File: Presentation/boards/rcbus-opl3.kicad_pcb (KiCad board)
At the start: 2 copper layers, 100 x 50 mm, 34 parts, among them CON1 SJ1-3523N, P1 RC2014 BUS, U1 74HCT688, U2 YMF262, U3 YAC512, U4 TL074, Y1 SG-8002CA

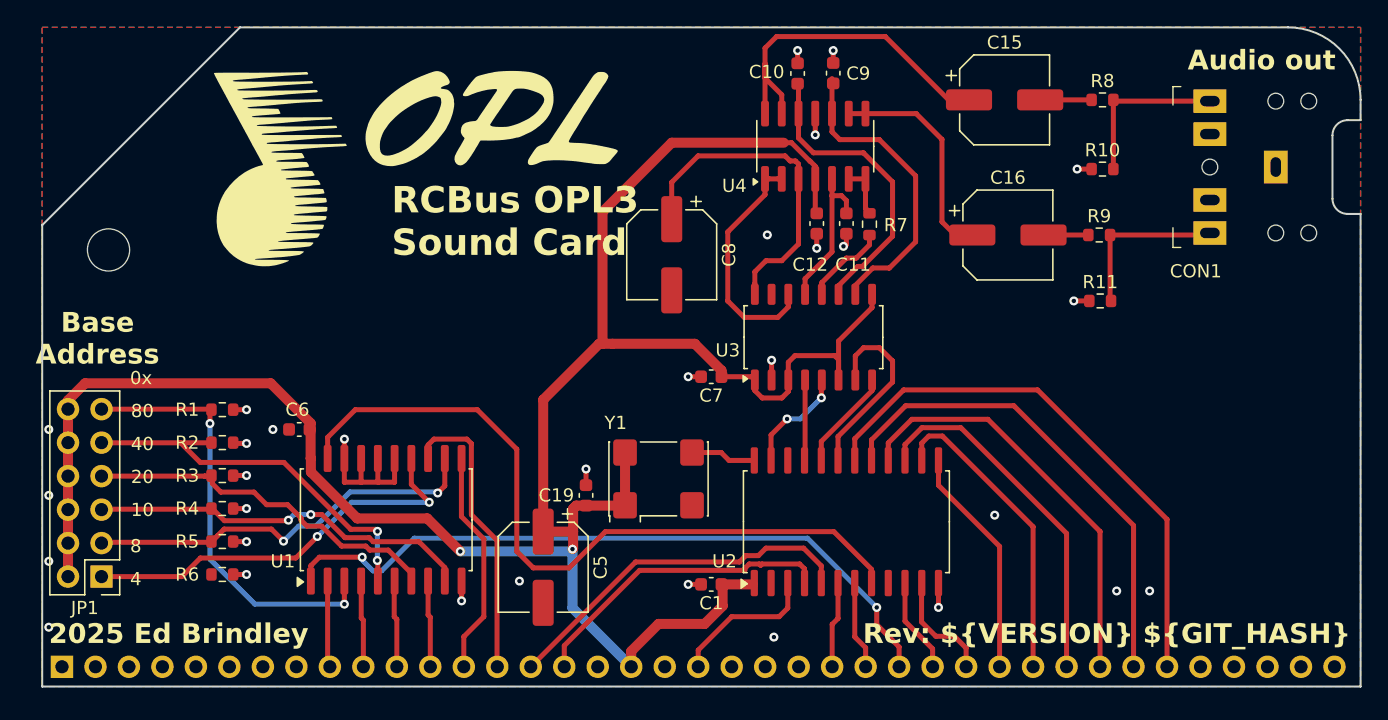
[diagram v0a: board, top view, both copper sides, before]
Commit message: Deploying to main from @ electrified/rcbus-opl3@95905a1b3d61b904a2086439a003ecc01cce0db1 🚀
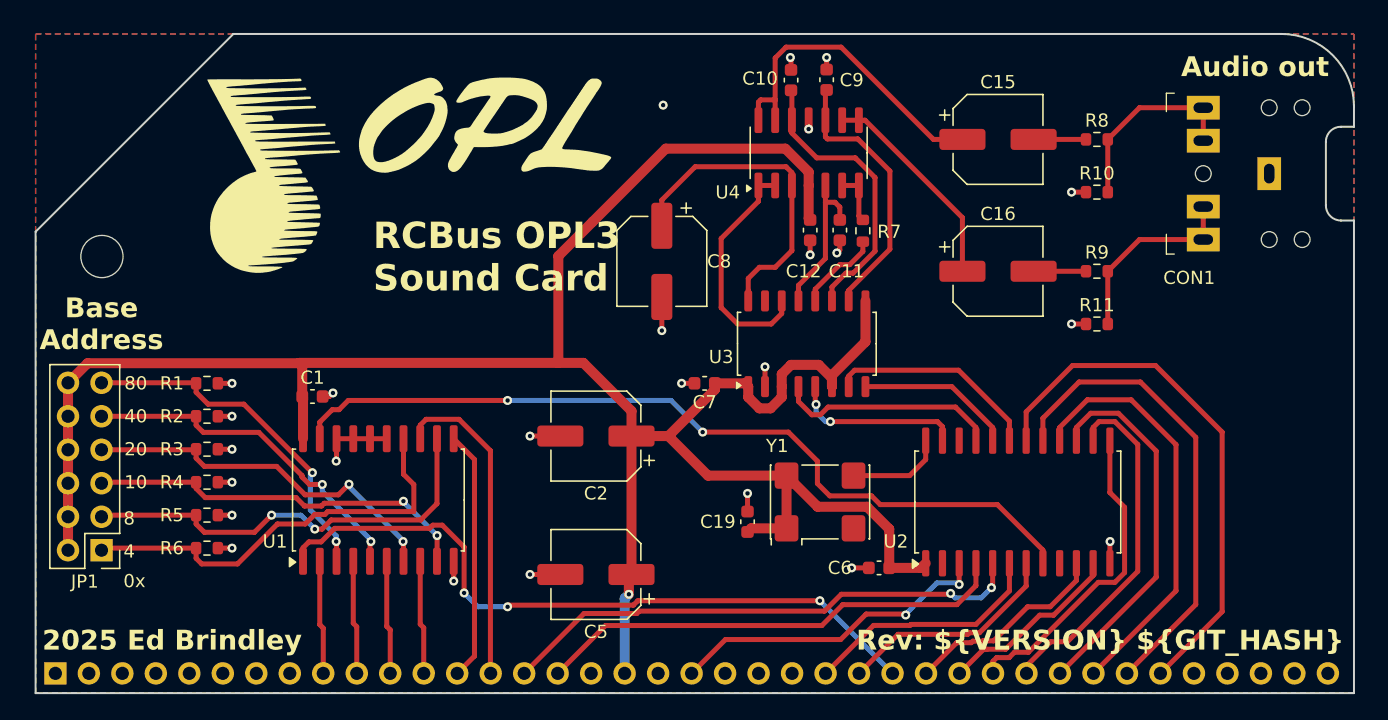
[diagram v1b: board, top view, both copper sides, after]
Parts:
- added C2: 10uf, Capacitor_SMD:CP_Elec_6.3x5.8, F.Cu at (102.5, 145.5)
- CON1: value SJ1-3523N -> 3.5mm jack
- Y1: value SG-8002CA -> 14.3181MHz
- moved C6 45.2 mm to (124.0, 155.5)
- moved C1 33.4 mm to (81.0, 142.5), turned to 0 degrees
- moved U2 13.1 mm to (134.5, 150.5)
- moved C19 12.4 mm to (114.0, 152.0)
- moved Y1 12.4 mm to (119.5, 150.5)
- moved C5 4.04 mm to (102.5, 156.0), turned to 180 degrees
- moved C15 3.04 mm to (133.0, 123.0)
- moved R8 3.03 mm to (140.5, 123.0)
- moved C16 2.85 mm to (133.0, 133.0)
- moved R9 2.76 mm to (140.5, 133.0)
- moved R1 2.31 mm to (73.0, 141.5)
- moved R2 2.31 mm to (73.0, 144.0)
- moved R3 2.31 mm to (73.0, 146.5)
- moved R4 2.31 mm to (73.0, 149.0)
- moved R5 2.31 mm to (73.0, 151.5)
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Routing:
- net /~{RESET}: track 11.0 -> 24.9 mm, vias 0 -> 2
- net /A1: track 27.6 -> 40.3 mm, vias 0 -> 2
- net /A0: track 23.8 -> 36.2 mm
- net /~{WR}: track 6.53 -> 18.6 mm
- net /DOAB: track 6.06 -> 16.9 mm
- net /~{RD}: track 6.69 -> 17.1 mm
- net /D0: track 7.22 -> 15.6 mm
- net /~{CS}: track 56.6 -> 63.5 mm, vias 0 -> 2
- net /D2: track 17.6 -> 24.2 mm
- net Net-(JP1-Pin_11): track 32.7 -> 26.8 mm
- net /D1: track 8.56 -> 14.1 mm
- net /DAC_CLK: track 8.23 -> 13.1 mm
- net /SMPAC: track 7.69 -> 11.9 mm
- net /D3: track 23.5 -> 26.9 mm
- net GND: track 31.6 -> 34.7 mm, vias 31 -> 25
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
